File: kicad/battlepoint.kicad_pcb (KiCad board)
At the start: 2 copper layers, 77.5 x 100.3 mm, 13 parts, among them J1 BTNS, P1 TMR1_LED, P10 OLED, P2 TMR2_LED, P3 CAP_LED, P4 OWN_LED, P5 SPK, P8 AUDIO_JACK, P9 KEYPAD, U1 DFPLAYER_MINI

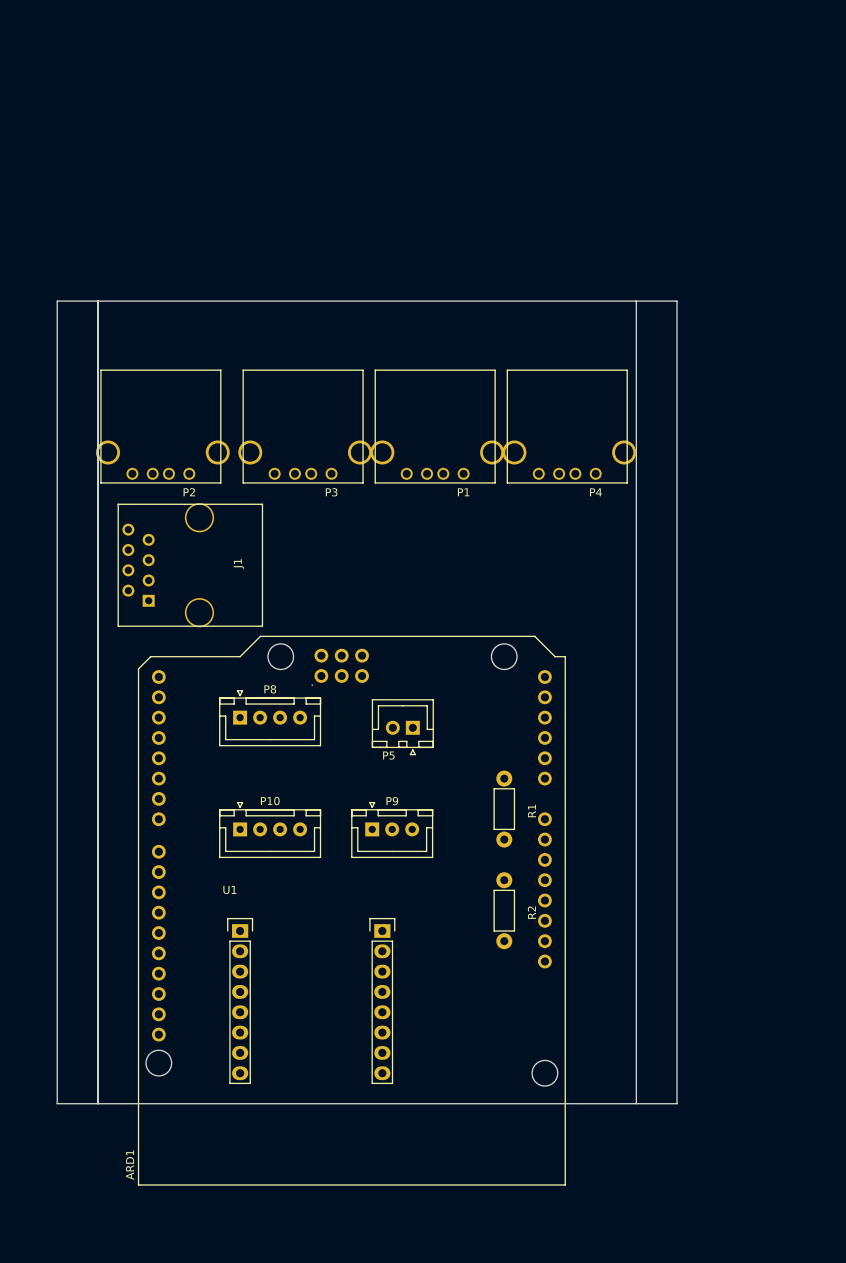
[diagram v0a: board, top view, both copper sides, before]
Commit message: progress
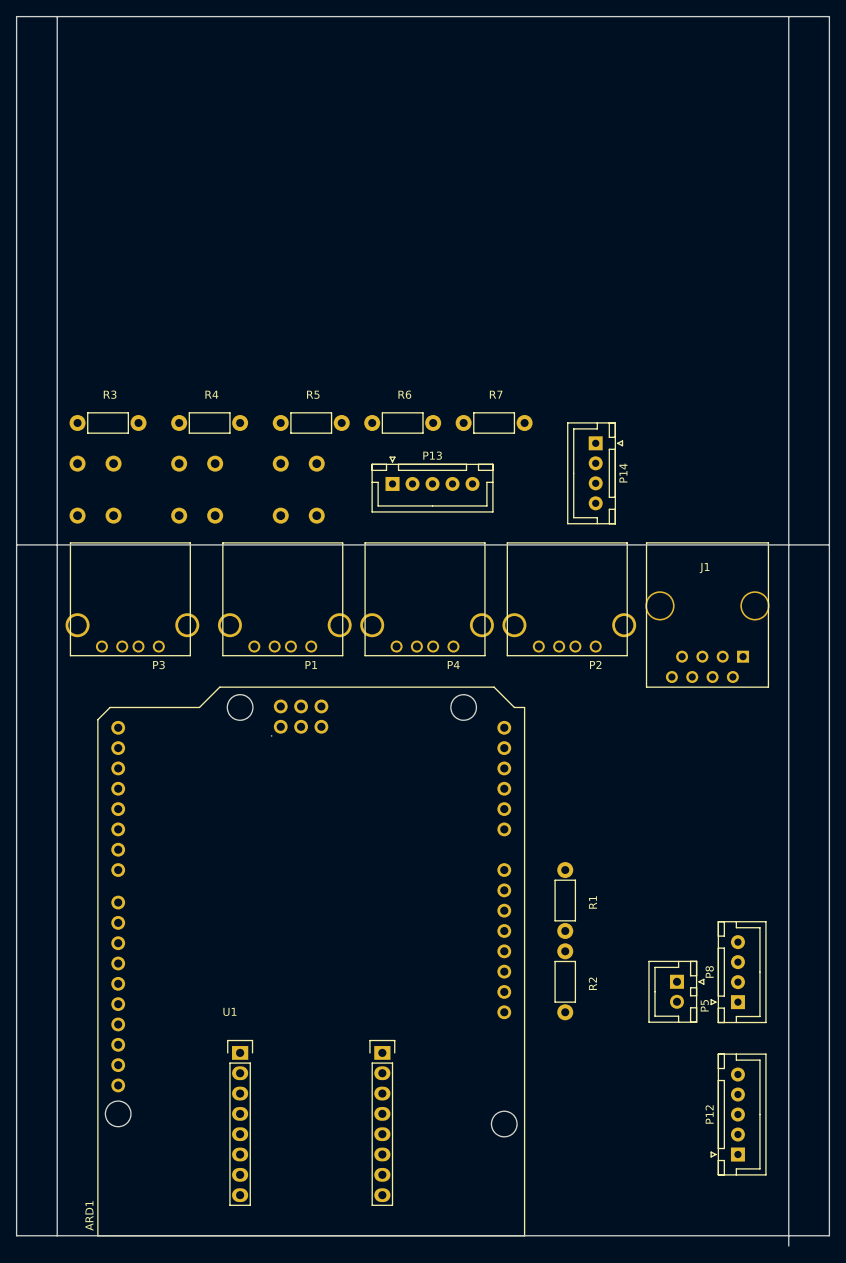
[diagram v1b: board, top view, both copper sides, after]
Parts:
- removed P10: OLED, Connectors_JST:JST_XH_B04B-XH-A_04x2.50mm_Straight
- removed P9: KEYPAD, Connectors_JST:JST_XH_B03B-XH-A_03x2.50mm_Straight
- added P12: PANEL_OUT, Connectors_JST:JST_XH_B05B-XH-A_05x2.50mm_Straight, F.Cu at (109.2, 184.2)
- added P13: PANEL_IN, Connectors_JST:JST_XH_B05B-XH-A_05x2.50mm_Straight, F.Cu at (66.0, 100.3)
- added P14: OLED_OUT, Connectors_JST:JST_XH_B04B-XH-A_04x2.50mm_Straight, F.Cu at (91.4, 95.2)
- added R3: 2K, Resistors_ThroughHole:Resistor_Horizontal_RM7mm, F.Cu at (26.7, 92.7)
- added R4: 330, Resistors_ThroughHole:Resistor_Horizontal_RM7mm, F.Cu at (39.4, 92.7)
- added R5: 620, Resistors_ThroughHole:Resistor_Horizontal_RM7mm, F.Cu at (52.1, 92.7)
- added R6: 1K, Resistors_ThroughHole:Resistor_Horizontal_RM7mm, F.Cu at (63.5, 92.7)
- added R7: 3.3K, Resistors_ThroughHole:Resistor_Horizontal_RM7mm, F.Cu at (74.9, 92.7)
- added SW1: BTN_UP, Buttons_Switches_ThroughHole:SW_PUSH_6mm, B.Cu at (26.7, 97.8)
- added SW2: BTN_DWN, Buttons_Switches_ThroughHole:SW_PUSH_6mm, B.Cu at (39.4, 97.8)
- added SW3: BTN_SEL, Buttons_Switches_ThroughHole:SW_PUSH_6mm, B.Cu at (52.1, 97.8)
- moved P8 71.7 mm to (109.2, 165.1), turned to 90 degrees
- moved J1 63.7 mm to (105.4, 115.6), turned to 180 degrees
- moved P2 55.2 mm to (91.4, 120.7)
- moved P5 45.8 mm to (101.6, 162.6), turned to 270 degrees
- moved P3 30.5 mm to (36.8, 120.7)
- moved P1 28.8 mm to (55.9, 120.7)
- moved P4 28.0 mm to (73.7, 120.7)
- moved U1 15.2 mm to (45.7, 171.4)
- moved R1 13.7 mm to (87.6, 148.6)
- moved R2 11.7 mm to (87.6, 158.8)
- moved ARD1 8.13 mm to (82.5, 194.3)
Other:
- board size 77.5 x 100.3 mm -> 101.6 x 153.7 mm
